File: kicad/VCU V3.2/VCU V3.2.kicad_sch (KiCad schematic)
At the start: 23 parts, among them J3 AVR-ISP-6, J4 Conn_01x03, J5 Conn_01x04, SW1 SW_Push, U1 ATmega328P-A, Y1 16MHz

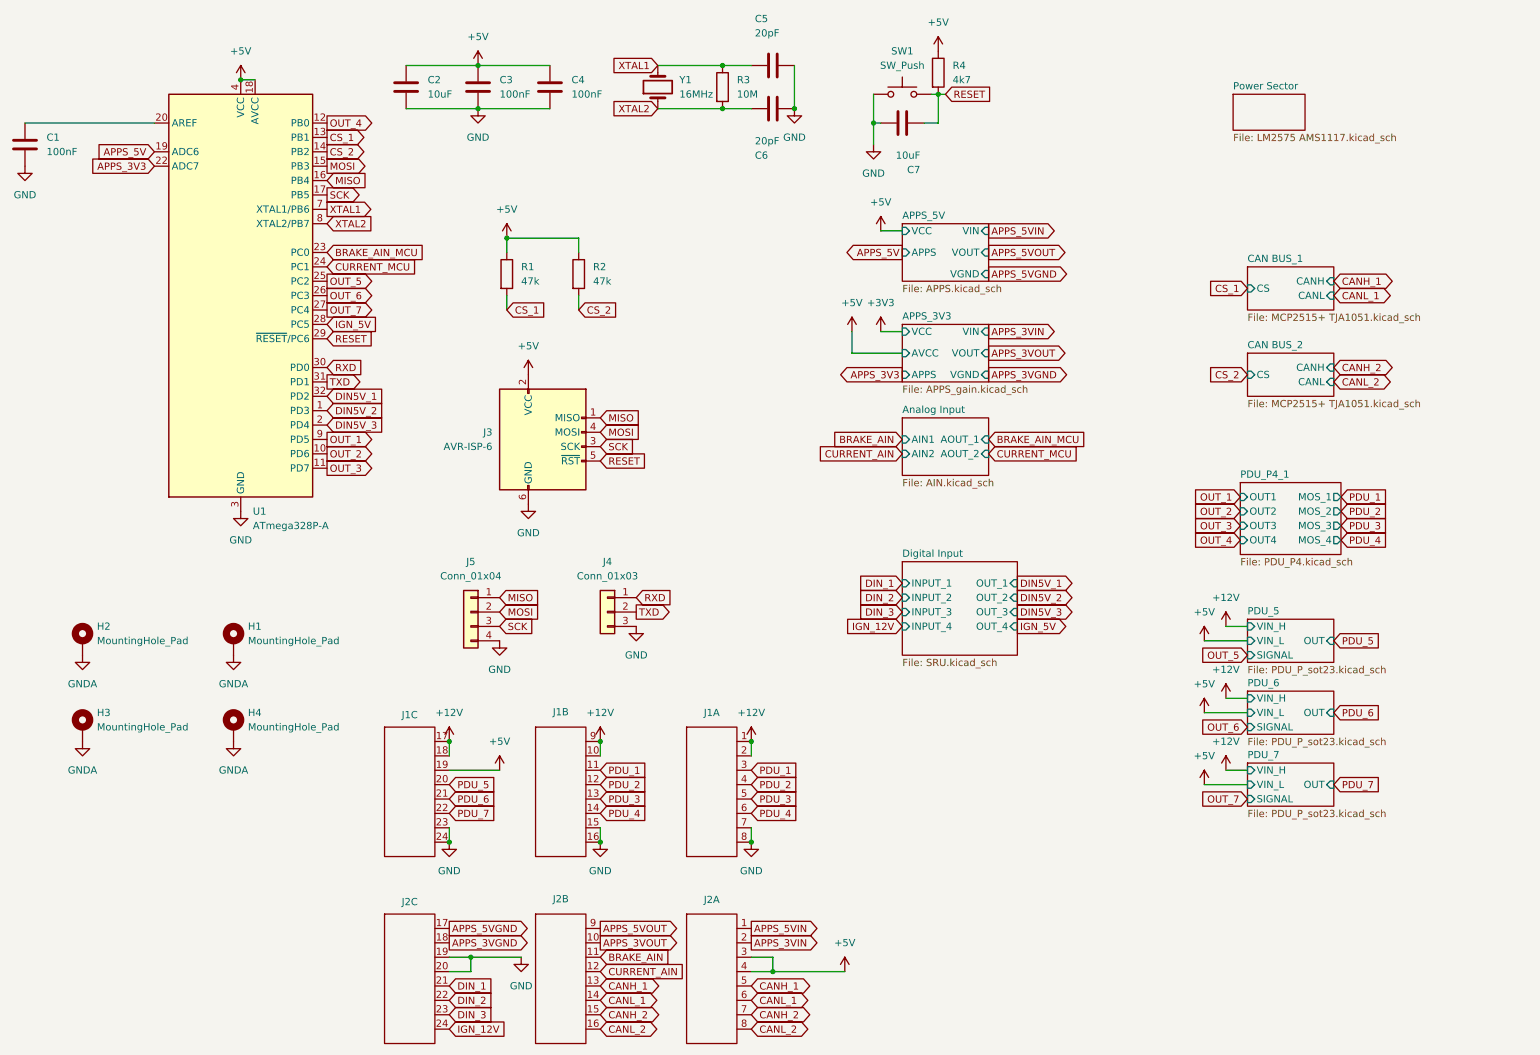
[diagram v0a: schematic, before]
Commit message: AHHHHH vcu v3.2
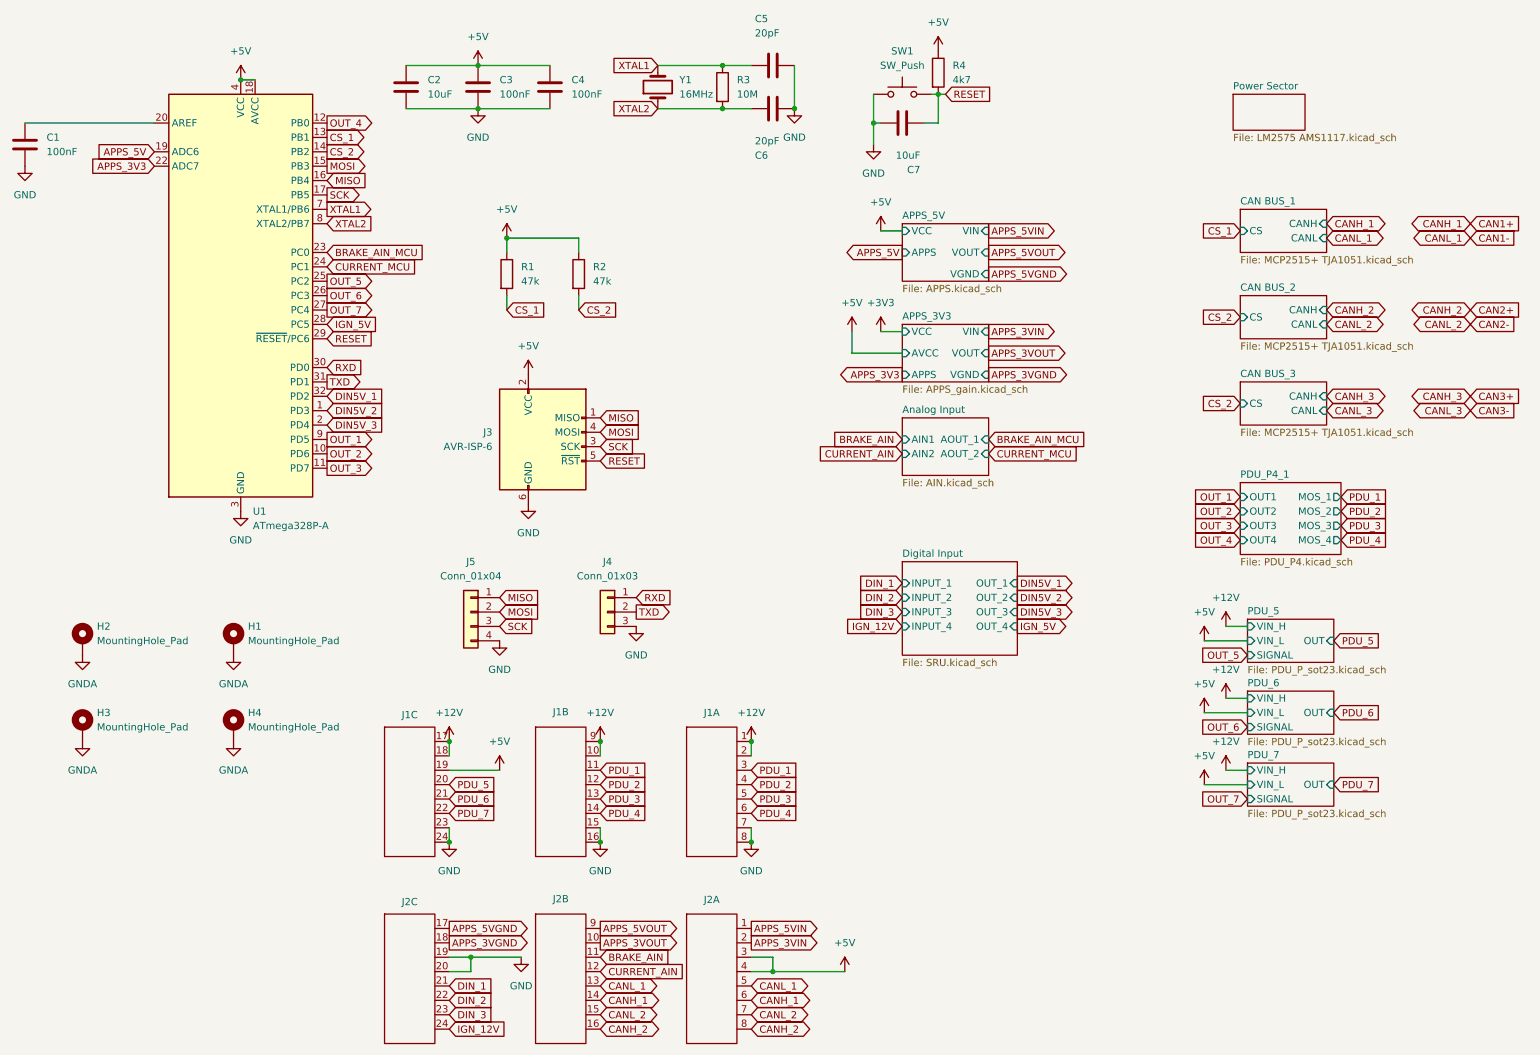
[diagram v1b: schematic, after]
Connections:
- net CANH_1 renamed CAN1-
- net CANH_2 renamed CAN2-
- net CANL_1 renamed CAN1+
- net CANL_2 renamed CAN2+
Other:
- added sheet CAN BUS_3 (MCP2515+ TJA1051.kicad_sch)

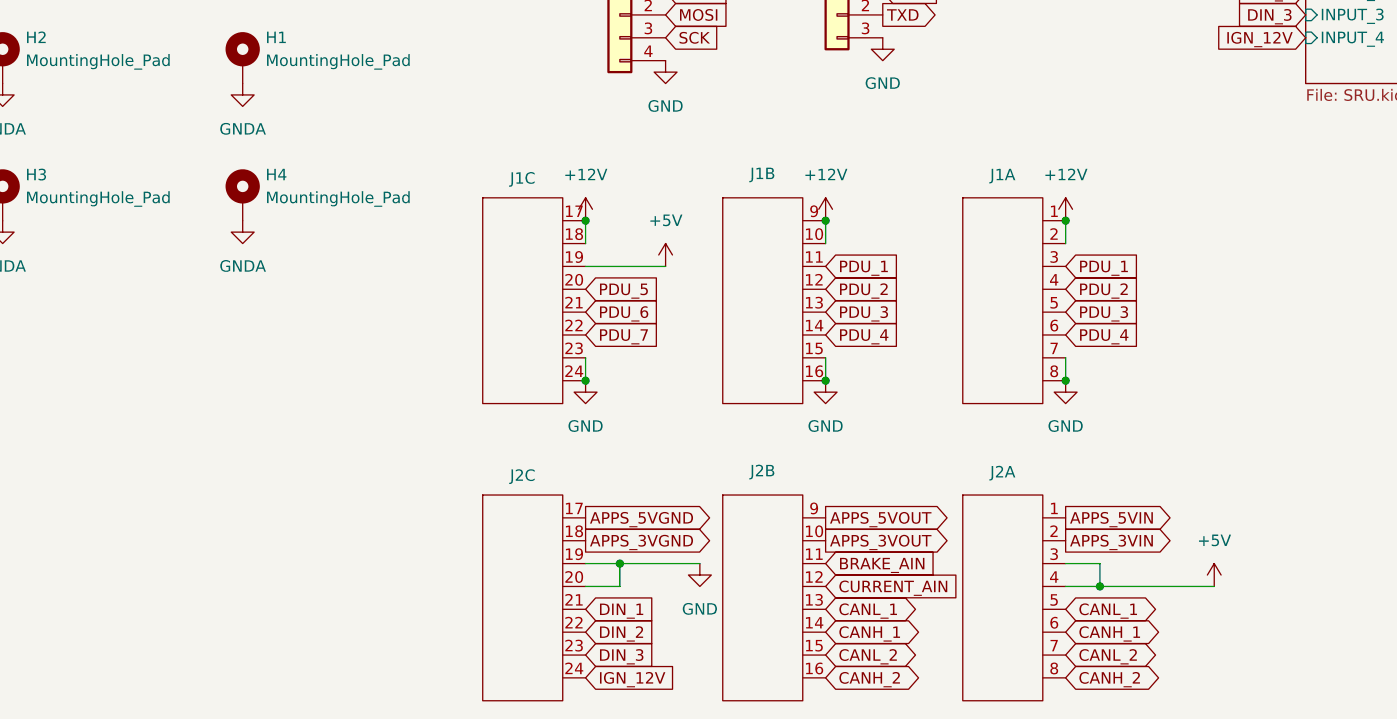
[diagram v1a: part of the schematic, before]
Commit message: haha VCU V3.2 AND NEW SCHEMATICS HAHAHA
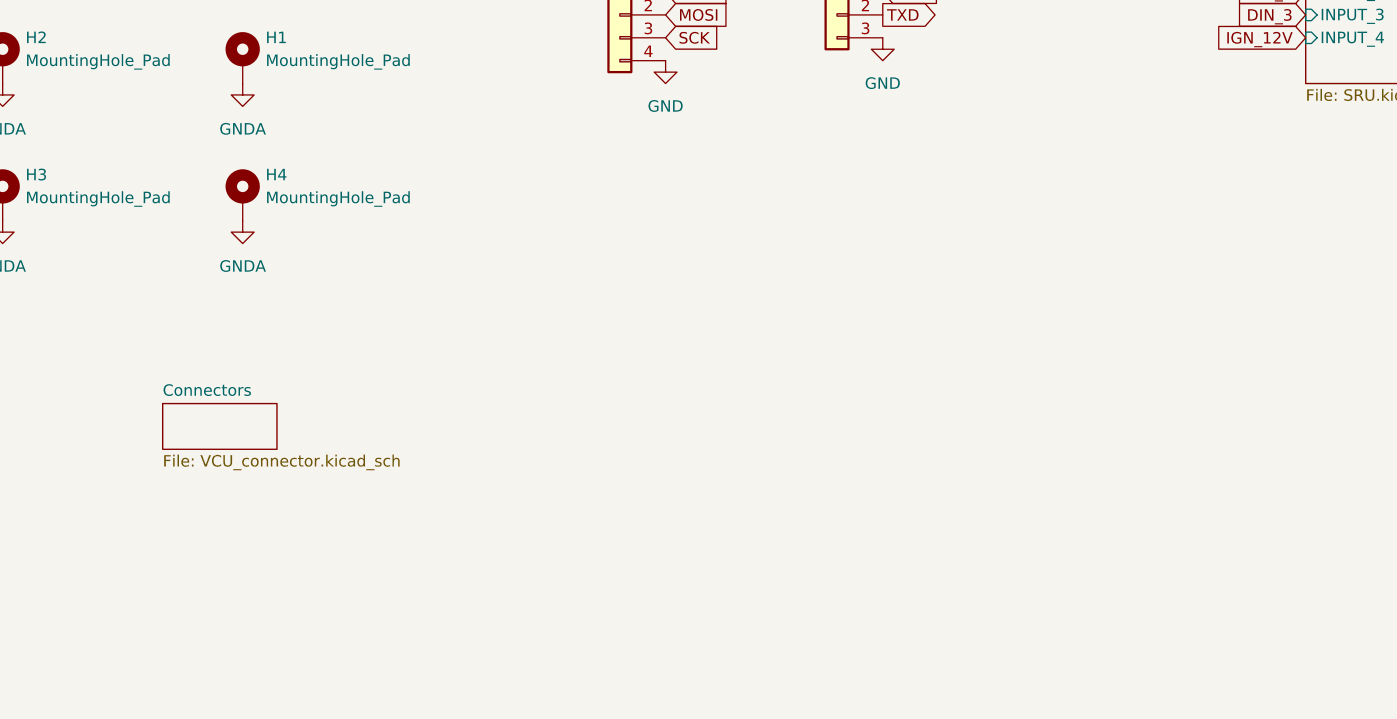
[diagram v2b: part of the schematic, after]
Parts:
- removed J1: ~, RMC_Connnector:HD241_24pin, symbol HD241:HD241
- removed J2: ~, RMC_Connnector:HD241_GF30, symbol HD241:HD241
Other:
- added sheet Connectors (VCU_connector.kicad_sch)
